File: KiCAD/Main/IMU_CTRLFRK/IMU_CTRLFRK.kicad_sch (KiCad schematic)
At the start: 12 parts, among them U7 BNO085, U8 VCNL4040M3OE, U9 BME280

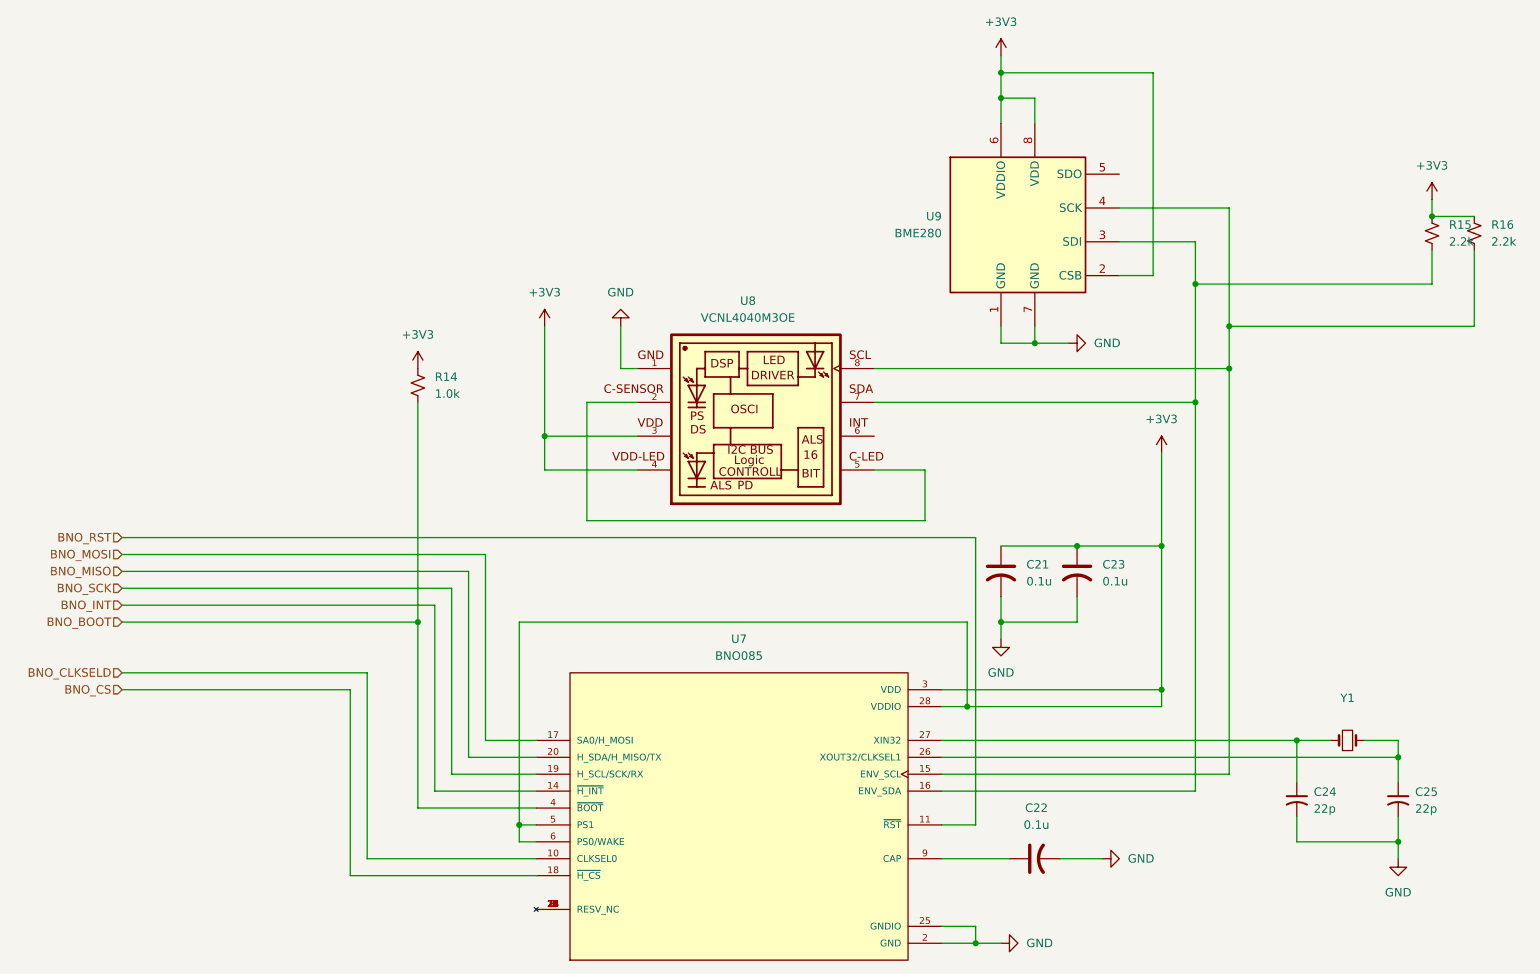
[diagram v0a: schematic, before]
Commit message: Submit design for review
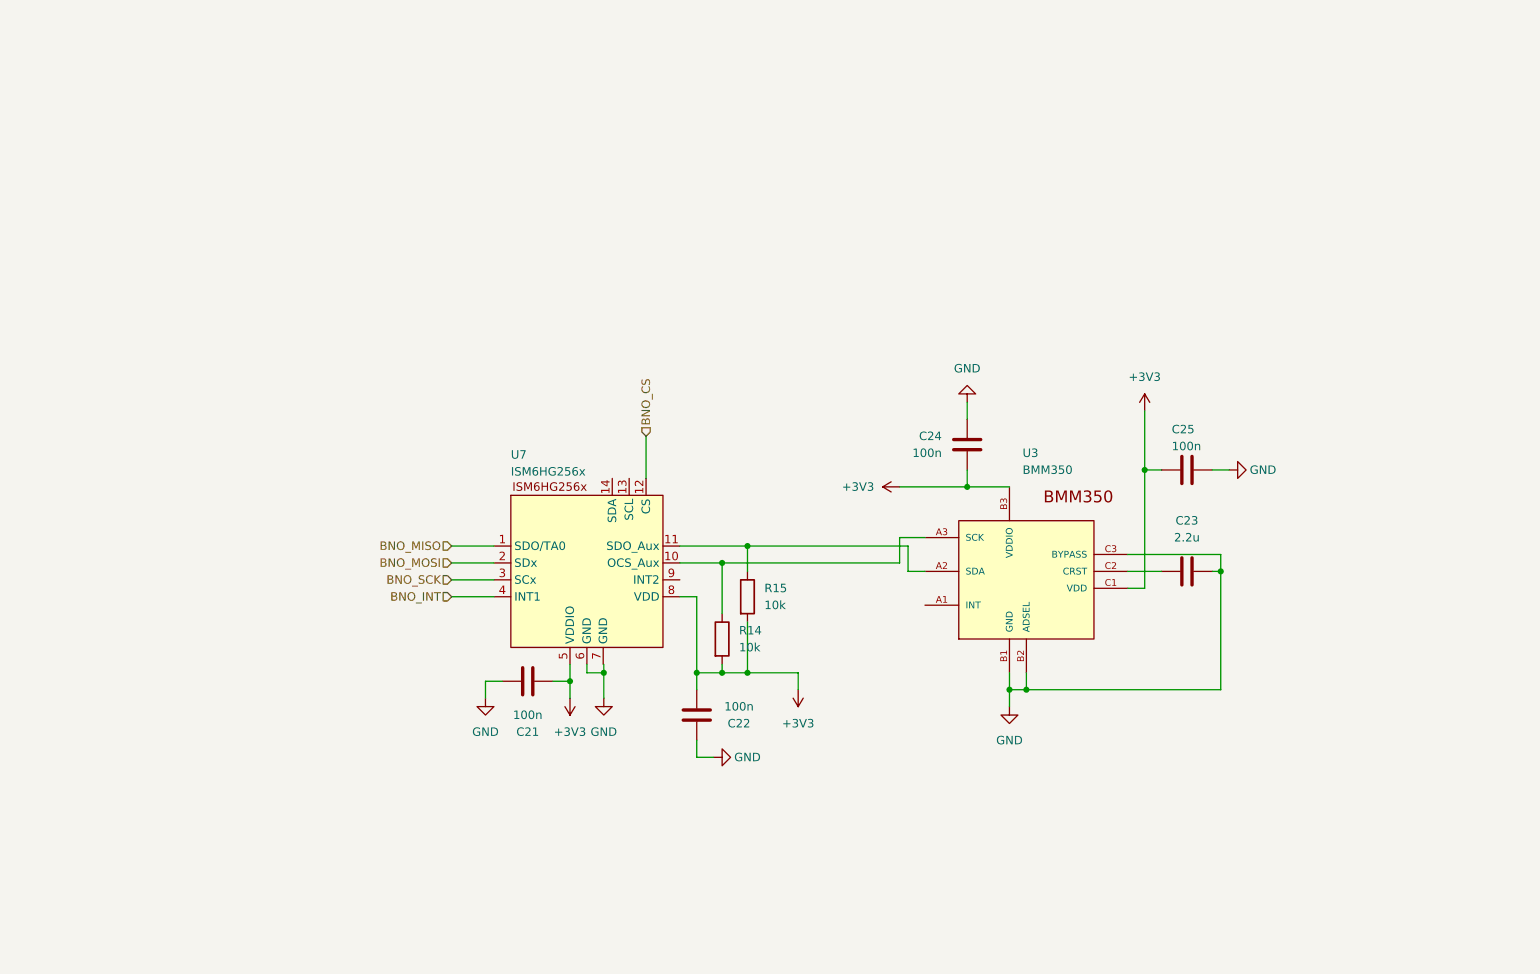
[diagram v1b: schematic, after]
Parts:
- removed C21, C22, C23: 0.1u, symbol Device:C_US
- removed C24, C25: 22p, symbol Device:C_Small_US
- removed R14: 1.0k, symbol Device:R_Small_US
- removed R15, R16: 2.2k, symbol Device:R_Small_US
- removed U7: BNO085, BNO085:IC_BNO085, symbol BNO085:BNO085
- removed U8: VCNL4040M3OE, VCNL4040M3OE:VISHAY_VCNL4040_4X2X1.1, symbol VCNL4040:VCNL4040M3OE
- removed U9: BME280, Package_LGA:Bosch_LGA-8_2.5x2.5mm_P0.65mm_ClockwisePinNumbering, symbol Sensor:BME280
- removed Y1: ~, symbol Device:Crystal_Small
- added C21, C22, C24, C25: 100n, symbol Device:C
- added C23: 2.2u, symbol Device:C
- added R14, R15: 10k, symbol Device:R
- added U3: BMM350, BMM350:BGA9C40P3X3_128X128X50, symbol BMM350:BMM350
- added U7: ISM6HG256x, symbol ISM6HG256XTR:ISM6HG256XTR
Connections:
- net +3V3: now also C21.2, C22.2, C24.2, C25.2, R14.2, R15.2, U3.B3 (VDDIO), U3.C1 (VDD), U7.5 (VDDIO), U7.8 (VDD)
- net BNO_CS: now also U7.12 (CS)
- net BNO_INT: now also U7.4 (INT1)
- net BNO_MISO: now also U7.1 (SDO/TA0)
- net BNO_MOSI: now also U7.2 (SDx)
- net BNO_SCK: now also U7.3 (SCx)
- net GND: now also C21.1, C22.1, C23.2, C24.1, C25.1, U3.B1 (GND), U3.B2 (ADSEL), U3.C3 (BYPASS), U7.6 (GND)
- new net: R15.1, U3.A2 (SDA), U7.11 (SDO_Aux)
- new net: R14.1, U3.A3 (SCK), U7.10 (OCS_Aux)
- new net: C23.1, U3.C2 (CRST)
